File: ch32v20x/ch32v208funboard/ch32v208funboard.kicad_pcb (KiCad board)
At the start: 2 copper layers, 40.6 x 35.6 mm, 22 parts, among them J1 HDR, J2 PGM, J3 USB_C_Receptacle_USB2.0, J4 HDR, U1 CH32V208GBU6, U3 XC6206P332, Y2 32MHz

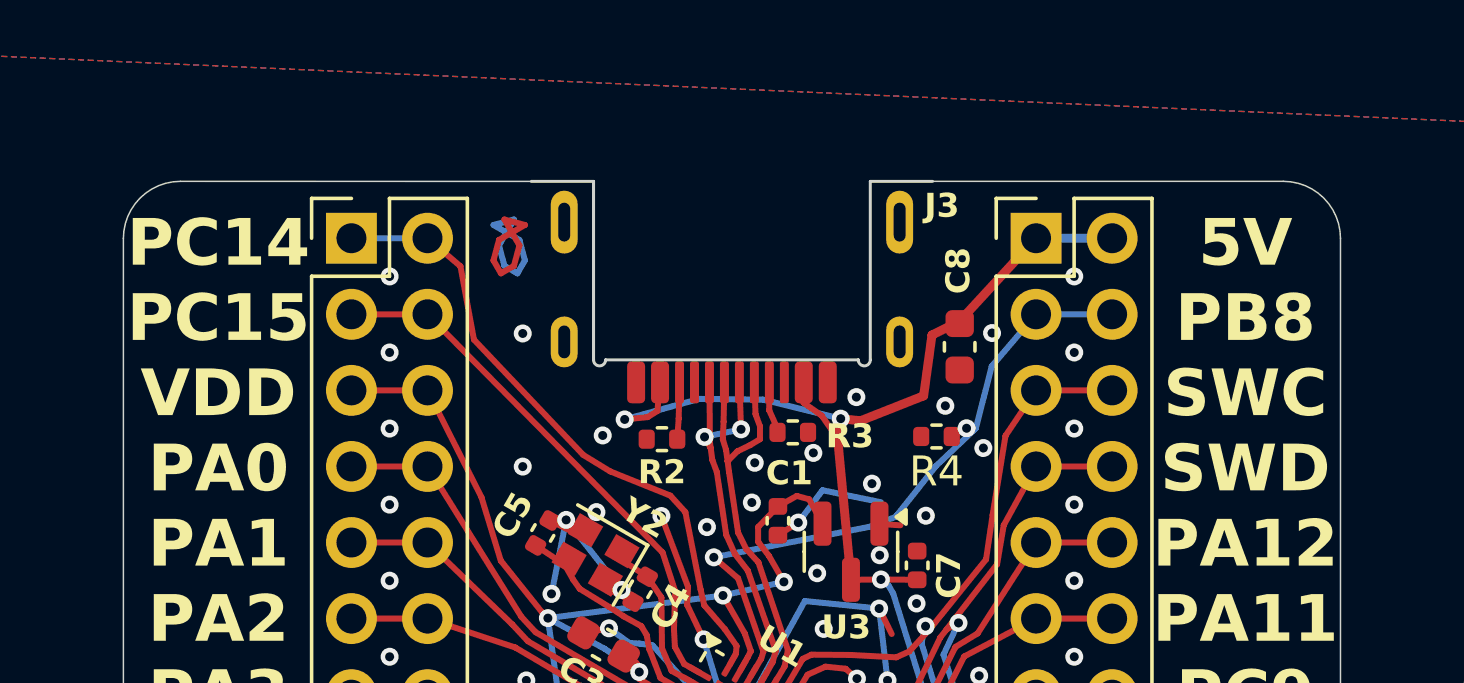
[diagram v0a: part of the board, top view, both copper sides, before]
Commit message: Bump funboards
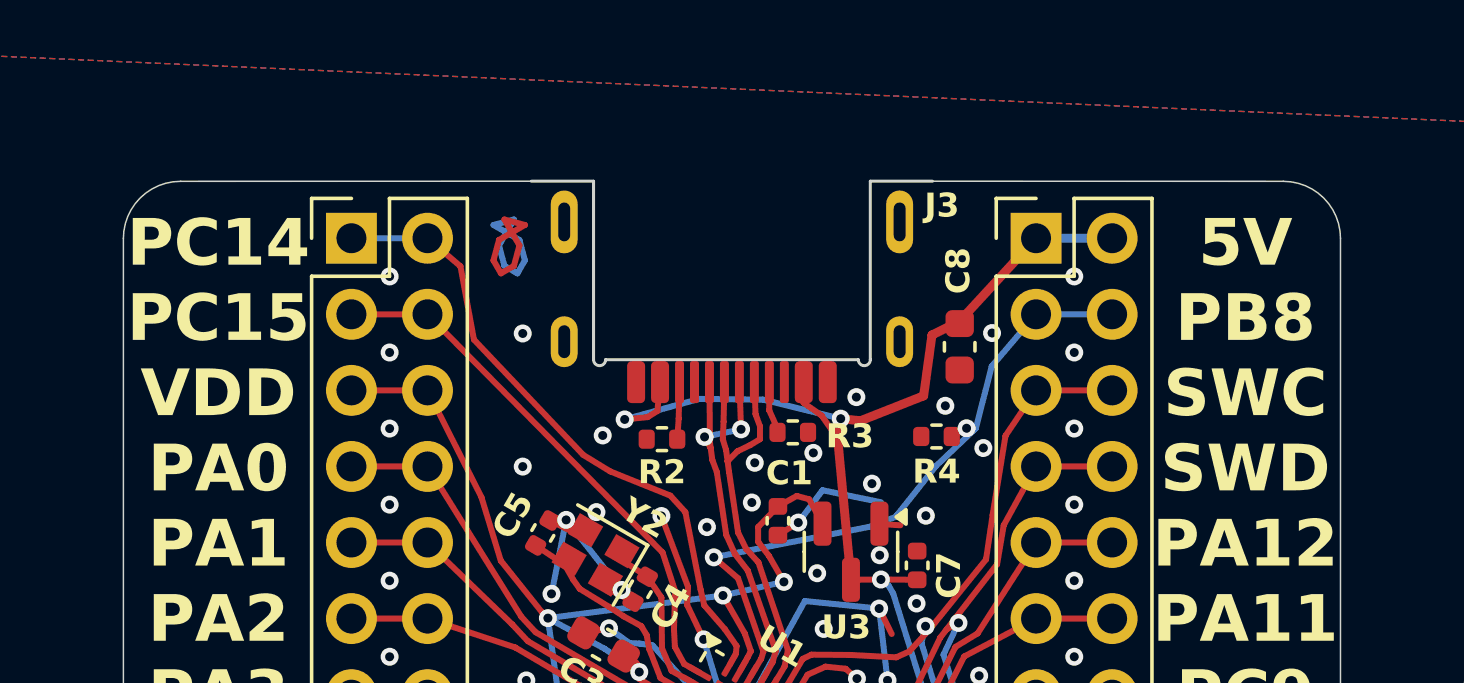
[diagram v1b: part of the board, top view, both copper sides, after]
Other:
- outline, holes or cut-outs redrawn
